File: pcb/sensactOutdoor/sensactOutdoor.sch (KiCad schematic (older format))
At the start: 118 parts, among them J1 48V, J10 CAN, J11 EXT2, J12 CAN, J13 RGB, J14 N1, J15 N2, J2 Conn_01x03, J3 Conn_01x03, J4 PROG, J5 LED CC, J6 PWM_OUT, J7 EXT1, J8 PWM_OUT, J9 230V, K1 ALDP105W, K2 ALDP105W, K3 ALDP105W, K4 ALDP105W, K5 ALDP105W, K6 ALDP105W, Q1 N, Q10 BC847, Q11 BC847, Q2 N, Q3 N, Q4 N, Q5 N, Q6 BC847, Q7 BC847, Q8 BC847, Q9 BC847, U1 ESP32-WROOM-32U, U2 A6211, U3 LMR16006X, U4 SN65HVD230, U5 AMS1117-3.3, U6 RF, U7 RX470B, U8 EL814

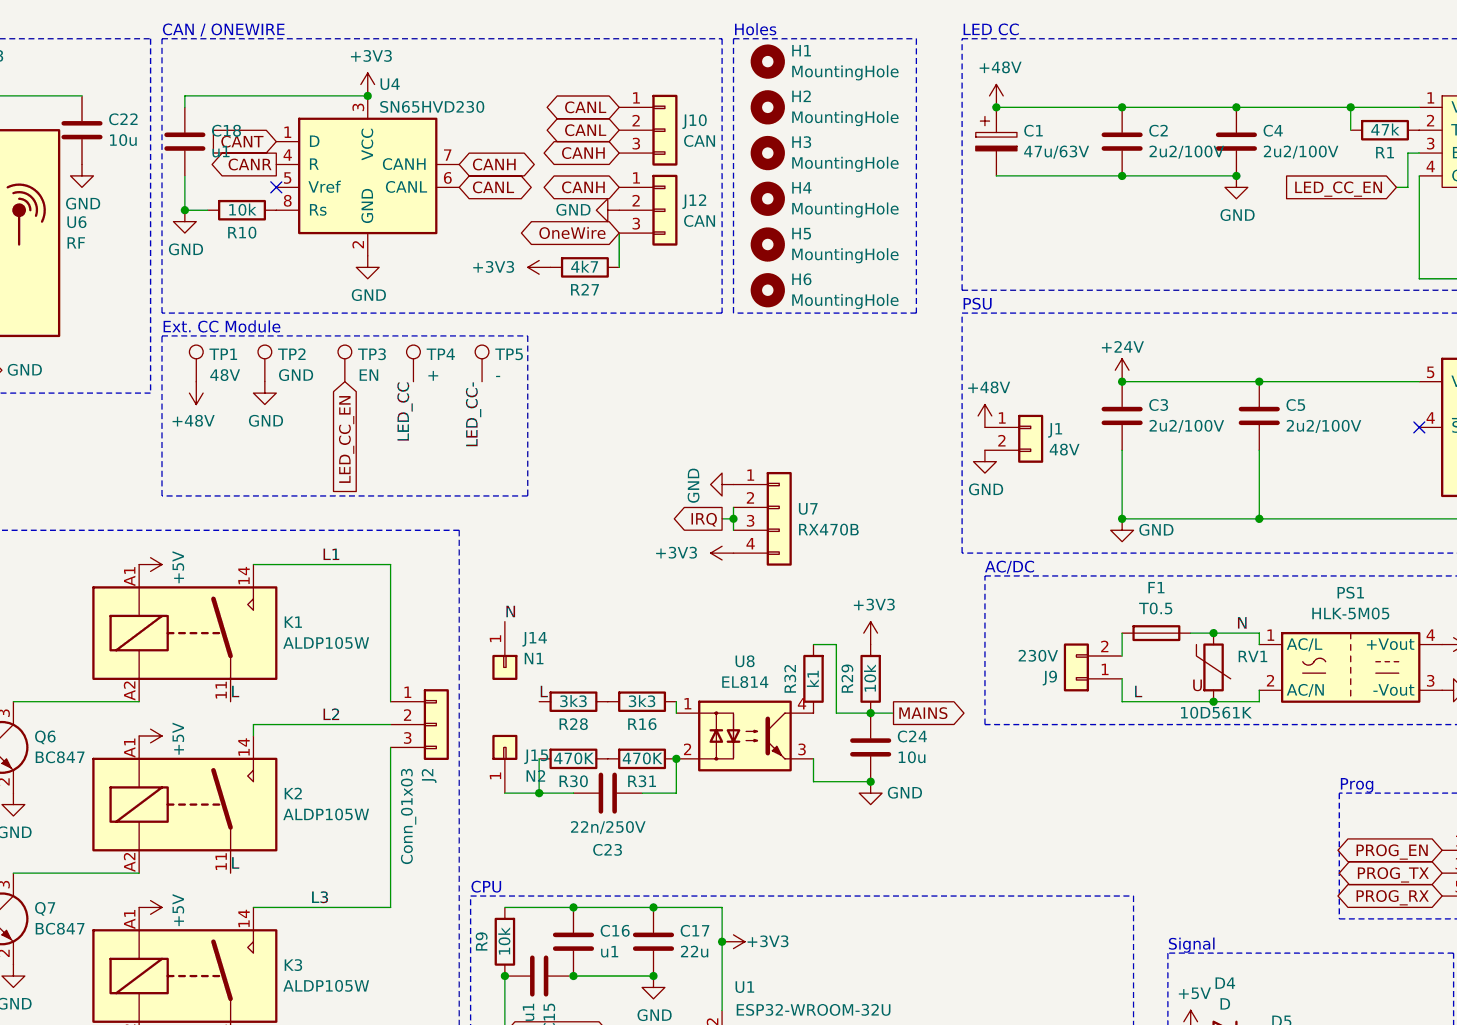
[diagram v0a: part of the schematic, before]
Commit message: variousChanges on sensactHSIO3+4 and sensactOutdoor
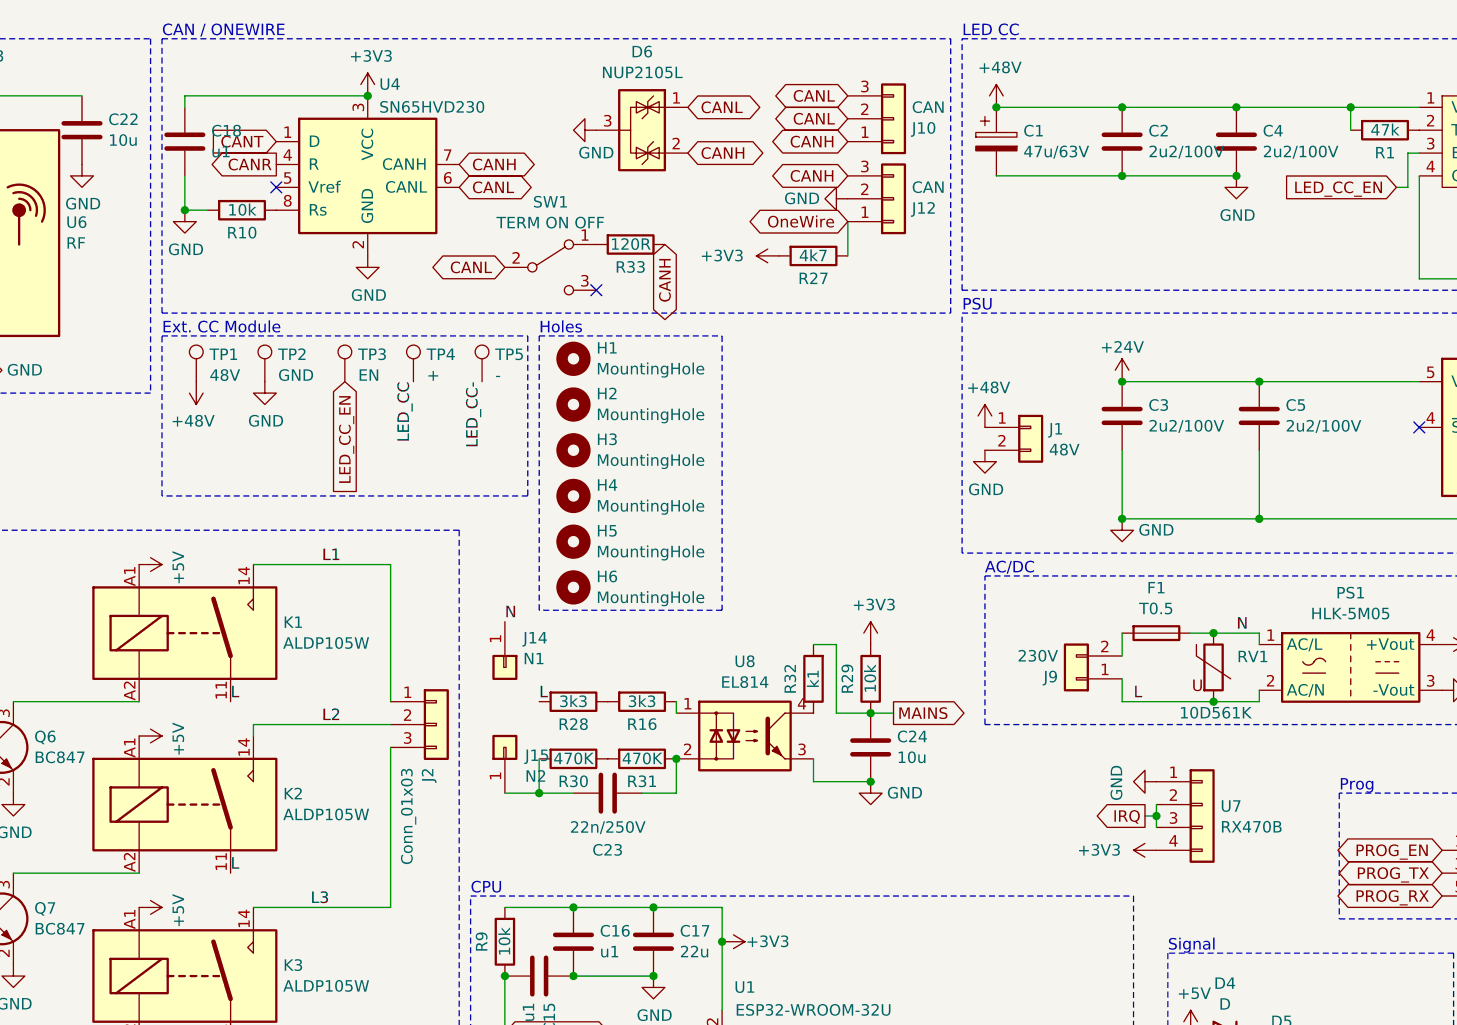
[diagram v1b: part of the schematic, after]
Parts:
- added D6: NUP2105L, Package_TO_SOT_SMD:SOT-23_Handsoldering, symbol Power_Protection:NUP2105L
- added R33: 120R, Resistor_SMD:R_1206_3216Metric_Pad1.30x1.75mm_HandSolder, symbol Device:R
- added SW1: TERM ON OFF, liebler_MECH:SW_SPDT_PCM12_handsolder, symbol Switch:SW_SPDT
- J10, J12, J13: footprint liebler_CONN:WAGO_250_203 -> liebler_CONN:KF250-3.5-3P-A
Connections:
- net CANH: now also J10.1 (Pin_1), J12.3 (Pin_3), D6.2 (K), R33.1; no longer J10.3 (Pin_3), J12.1 (Pin_1)
- net CANL: now also J10.3 (Pin_3), D6.1 (K), SW1.2 (B); no longer J10.1 (Pin_1)
- net GND: now also D6.3 (A)
- net OneWire: now also J12.1 (Pin_1); no longer J12.3 (Pin_3)
- new net: R33.2, SW1.1 (A)
- no-connect marks 8 -> 9
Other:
- moved on the sheet: H1, H2, H3, H4, H5, H6, J10, J12, R27, U7
